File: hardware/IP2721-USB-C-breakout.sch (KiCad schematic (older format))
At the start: 13 parts, among them J1 Conn_01x02_Female, Q1 AO3400A, U1 IP2721, U2 USB_C_PD_CONNECTOR

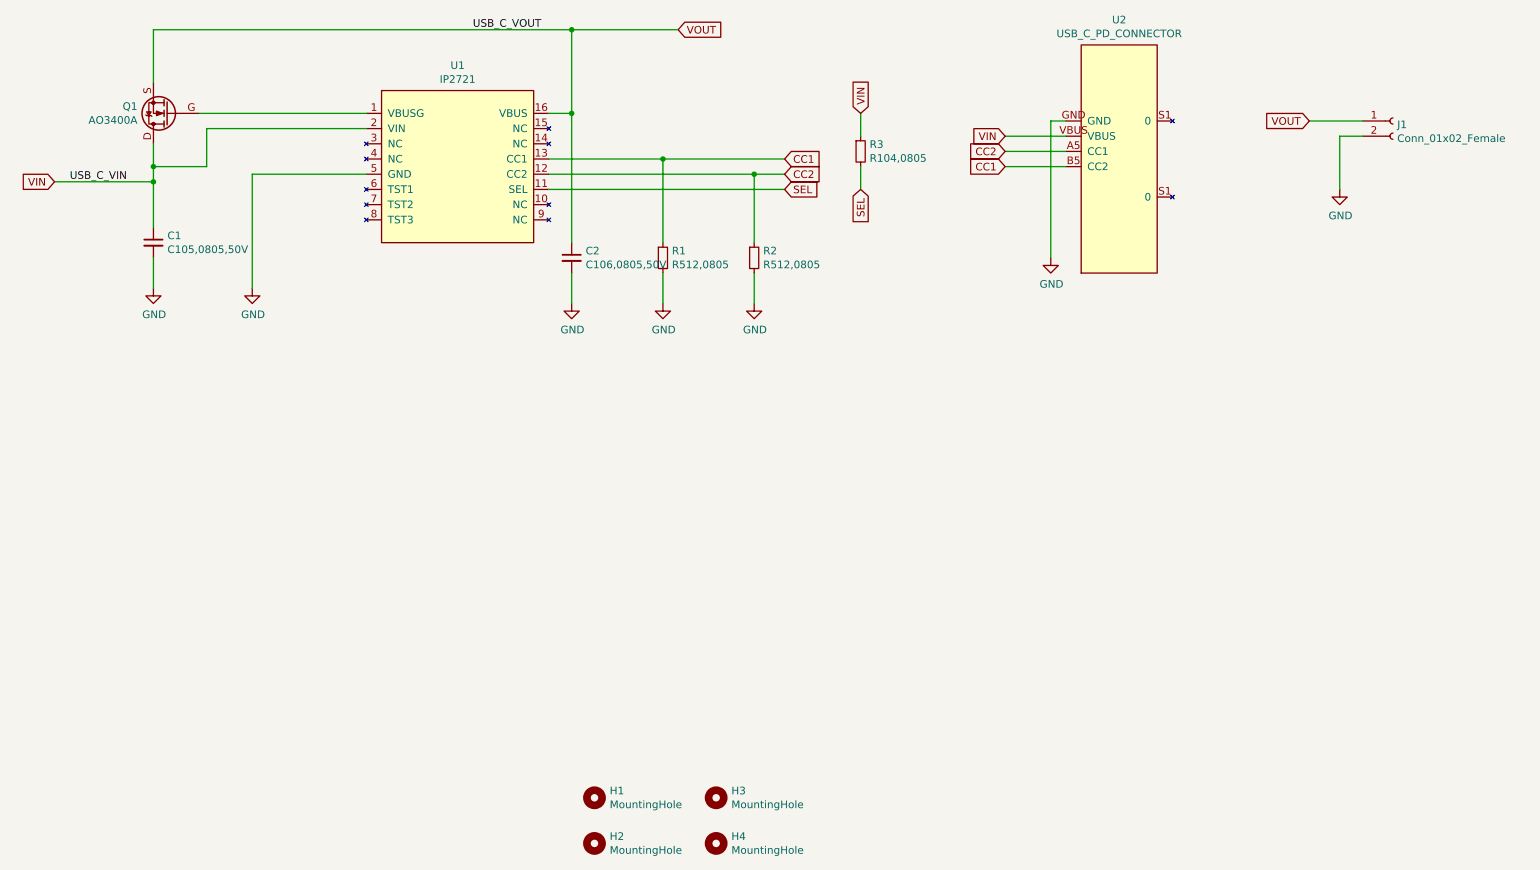
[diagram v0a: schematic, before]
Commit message: update and test,
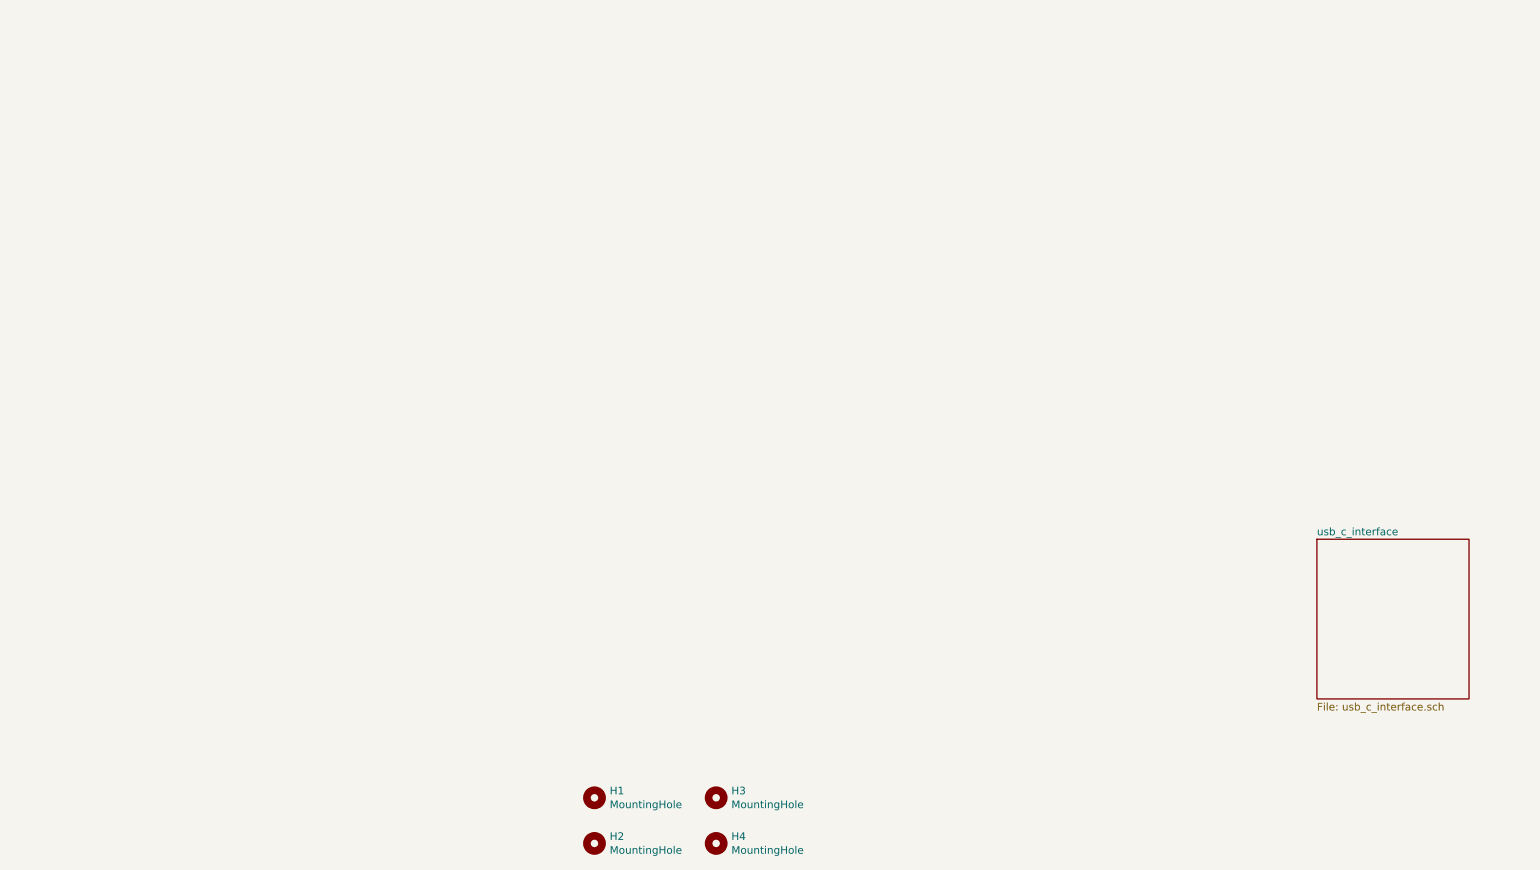
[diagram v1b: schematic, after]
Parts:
- removed C1: C105,0805,50V, Capacitor_SMD:C_0805_2012Metric_Pad1.18x1.45mm_HandSolder, symbol taobao-c:C106,0805
- removed C2: C106,0805,50V, Capacitor_SMD:C_0805_2012Metric_Pad1.18x1.45mm_HandSolder, symbol taobao-c:C105,0805
- removed J1: Conn_01x02_Female, Connector_PinHeader_2.54mm:PinHeader_1x02_P2.54mm_Vertical, symbol Connector:Conn_01x02_Female
- removed Q1: AO3400A, footprint:AO3400,SOT23, symbol taobao-transistor:AO3400A
- removed R1, R2: R512,0805, Resistor_SMD:R_0805_2012Metric_Pad1.20x1.40mm_HandSolder, symbol taobao-r:R513,0805
- removed R3: R104,0805, Resistor_SMD:R_0805_2012Metric_Pad1.20x1.40mm_HandSolder, symbol taobao-r:R104,0805
- removed U1: IP2721, Package_SO:TSSOP-16_4.4x5mm_P0.65mm, symbol IP2721-USB-C-breakout:IP2721
- removed U2: USB_C_PD_CONNECTOR, footprint:USBC_16PIN, symbol IP2721-USB-C-breakout:USB_C_PD_CONNECTOR
